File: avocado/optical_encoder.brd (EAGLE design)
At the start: 18.5 x 16.5 mm, 13 parts

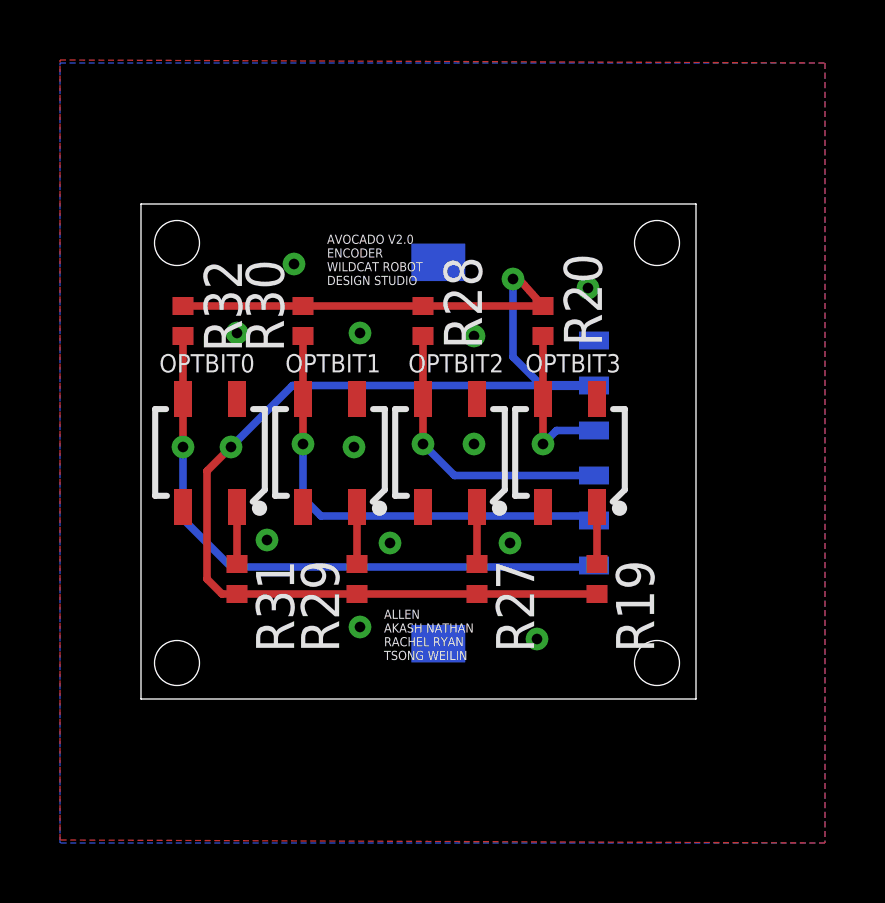
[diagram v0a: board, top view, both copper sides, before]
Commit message: version 2 of the avocado pcb finished
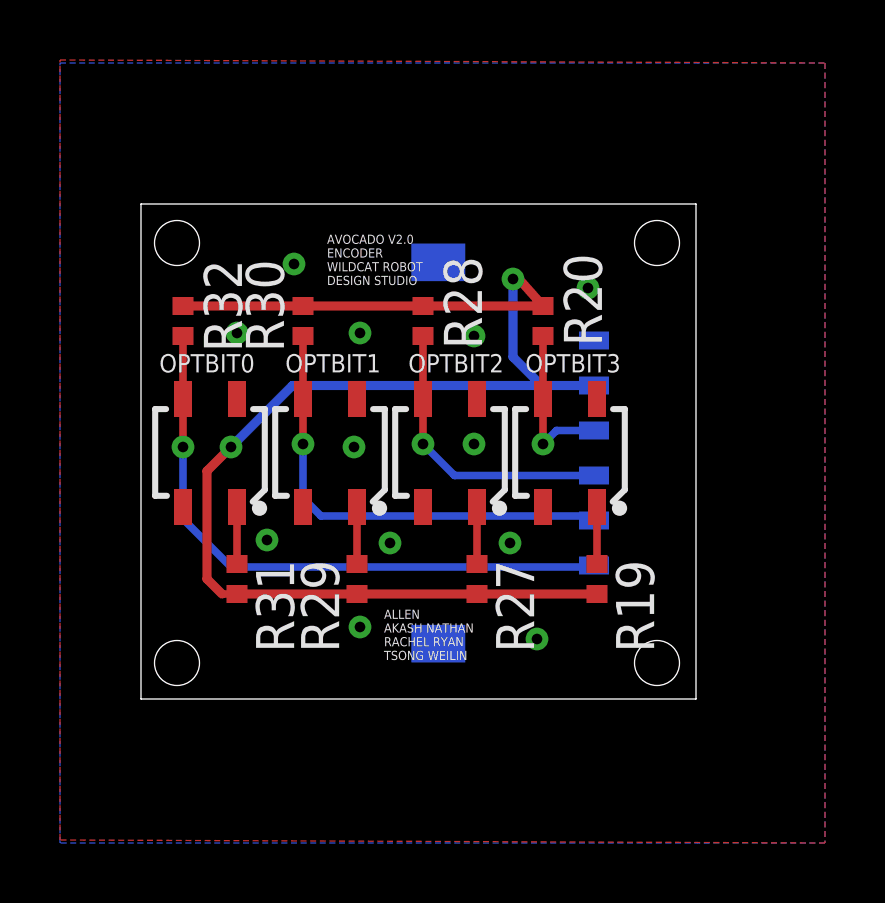
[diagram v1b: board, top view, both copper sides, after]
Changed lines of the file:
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@@
 <setting verticaltext="up"/>
 </settings>
-<grid distance="0.0999999999" unitdist="mm" unit="mm" style="lines" multiple="1" display="no" altdistance="5" altunitdist="mil" altunit="mil"/>
+<grid distance="3.93700787" unitdist="mil" unit="mil" style="lines" multiple="1" display="no" altdistance="5" altunitdist="mil" altunit="mil"/>
 <layers>
 <layer number="1" name="Top" color="4" fill="1" visible="yes" active="yes"/>
@@
 <contactref element="R31" pad="2"/>
 <contactref element="U$1" pad="5"/>
-<wire x1="2.6" y1="17.9" x2="6.6" y2="17.9" width="0.254" layer="1"/>
-<wire x1="4.4" y1="8.3" x2="8.4" y2="8.3" width="0.254" layer="1"/>
-<wire x1="8.4" y1="8.3" x2="12.4" y2="8.3" width="0.254" layer="1"/>
-<wire x1="12.4" y1="8.3" x2="16.4" y2="8.3" width="0.254" layer="1"/>
-<wire x1="6.6" y1="17.9" x2="10.6" y2="17.9" width="0.254" layer="1"/>
-<wire x1="10.6" y1="17.9" x2="14.6" y2="17.9" width="0.254" layer="1"/>
-<wire x1="14.6" y1="17.9" x2="13.8" y2="18.8" width="0.254" layer="1"/>
+<wire x1="2.6" y1="17.9" x2="6.6" y2="17.9" width="0.3048" layer="1"/>
+<wire x1="4.4" y1="8.3" x2="8.4" y2="8.3" width="0.3048" layer="1"/>
+<wire x1="8.4" y1="8.3" x2="12.4" y2="8.3" width="0.3048" layer="1"/>
+<wire x1="12.4" y1="8.3" x2="16.4" y2="8.3" width="0.3048" layer="1"/>
+<wire x1="6.6" y1="17.9" x2="10.6" y2="17.9" width="0.3048" layer="1"/>
+<wire x1="10.6" y1="17.9" x2="14.6" y2="17.9" width="0.3048" layer="1"/>
+<wire x1="14.6" y1="17.9" x2="13.8" y2="18.8" width="0.3048" layer="1"/>
 <wire x1="13.8" y1="18.8" x2="13.6" y2="18.8" width="0.254" layer="1"/>
 <via x="13.6" y="18.8" extent="1-16" drill="0.35"/>
-<wire x1="13.6" y1="18.8" x2="13.6" y2="16.2" width="0.254" layer="16"/>
+<wire x1="13.6" y1="18.8" x2="13.6" y2="16.2" width="0.3048" layer="16"/>
 <wire x1="4.4" y1="8.3" x2="3.9" y2="8.3" width="0.254" layer="1"/>
-<wire x1="3.9" y1="8.3" x2="3.4" y2="8.8" width="0.254" layer="1"/>
-<wire x1="3.4" y1="8.8" x2="3.4" y2="12.4" width="0.254" layer="1"/>
-<wire x1="3.4" y1="12.4" x2="4.2" y2="13.2" width="0.254" layer="1"/>
+<wire x1="3.9" y1="8.3" x2="3.4" y2="8.8" width="0.3048" layer="1"/>
+<wire x1="3.4" y1="8.8" x2="3.4" y2="12.4" width="0.3048" layer="1"/>
+<wire x1="3.4" y1="12.4" x2="4.2" y2="13.2" width="0.3048" layer="1"/>
 <via x="4.2" y="13.2" extent="1-16" drill="0.35"/>
-<wire x1="4.2" y1="13.2" x2="6.25" y2="15.25" width="0.254" layer="16"/>
-<wire x1="6.25" y1="15.25" x2="14.55" y2="15.25" width="0.254" layer="16"/>
+<wire x1="4.2" y1="13.2" x2="6.25" y2="15.25" width="0.3048" layer="16"/>
+<wire x1="6.25" y1="15.25" x2="14.55" y2="15.25" width="0.3048" layer="16"/>
 <wire x1="14.7" y1="15.25" x2="16.3" y2="15.25" width="0.3048" layer="16"/>
-<wire x1="13.6" y1="16.2" x2="14.55" y2="15.25" width="0.254" layer="16"/>
+<wire x1="13.6" y1="16.2" x2="14.55" y2="15.25" width="0.3048" layer="16"/>
 <wire x1="14.55" y1="15.25" x2="14.7" y2="15.25" width="0.254" layer="16"/>
 </signal>
